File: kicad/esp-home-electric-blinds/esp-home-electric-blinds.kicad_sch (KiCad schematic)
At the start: 10 parts, among them J1 AC_IN, J2 Stepper_2_conn, J3 Stepper_2_conn, J4 Conn_01x05, U1 ESP32_mini, U2 TMC2208_Stepper_driver, U3 TMC2208_Stepper_driver

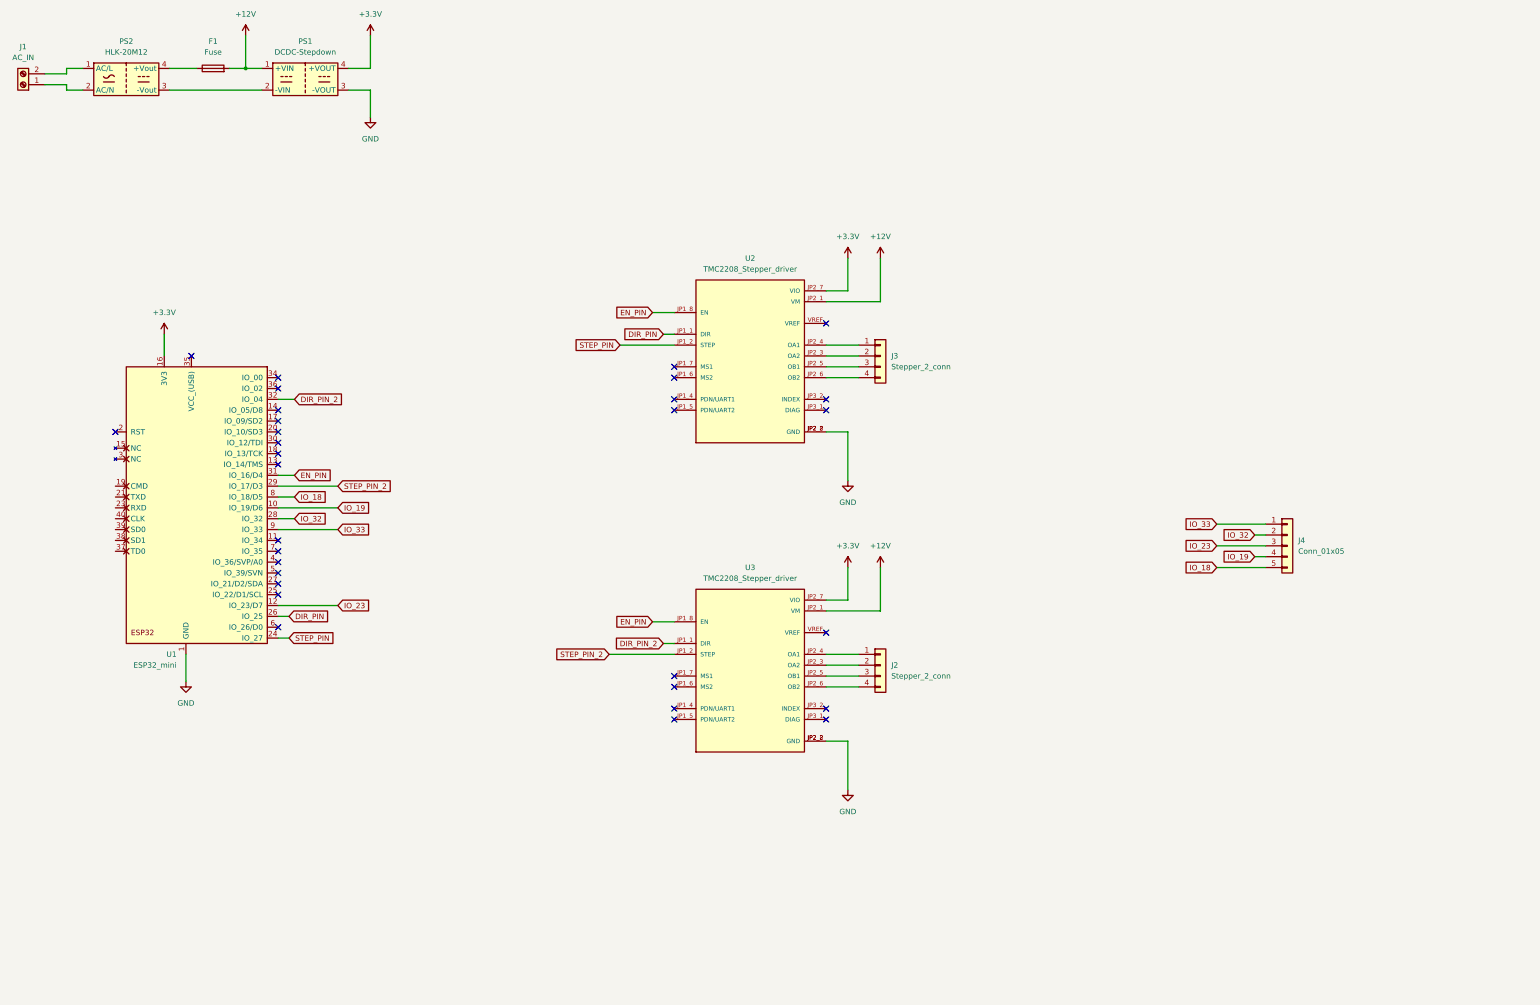
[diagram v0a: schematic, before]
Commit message: rearange
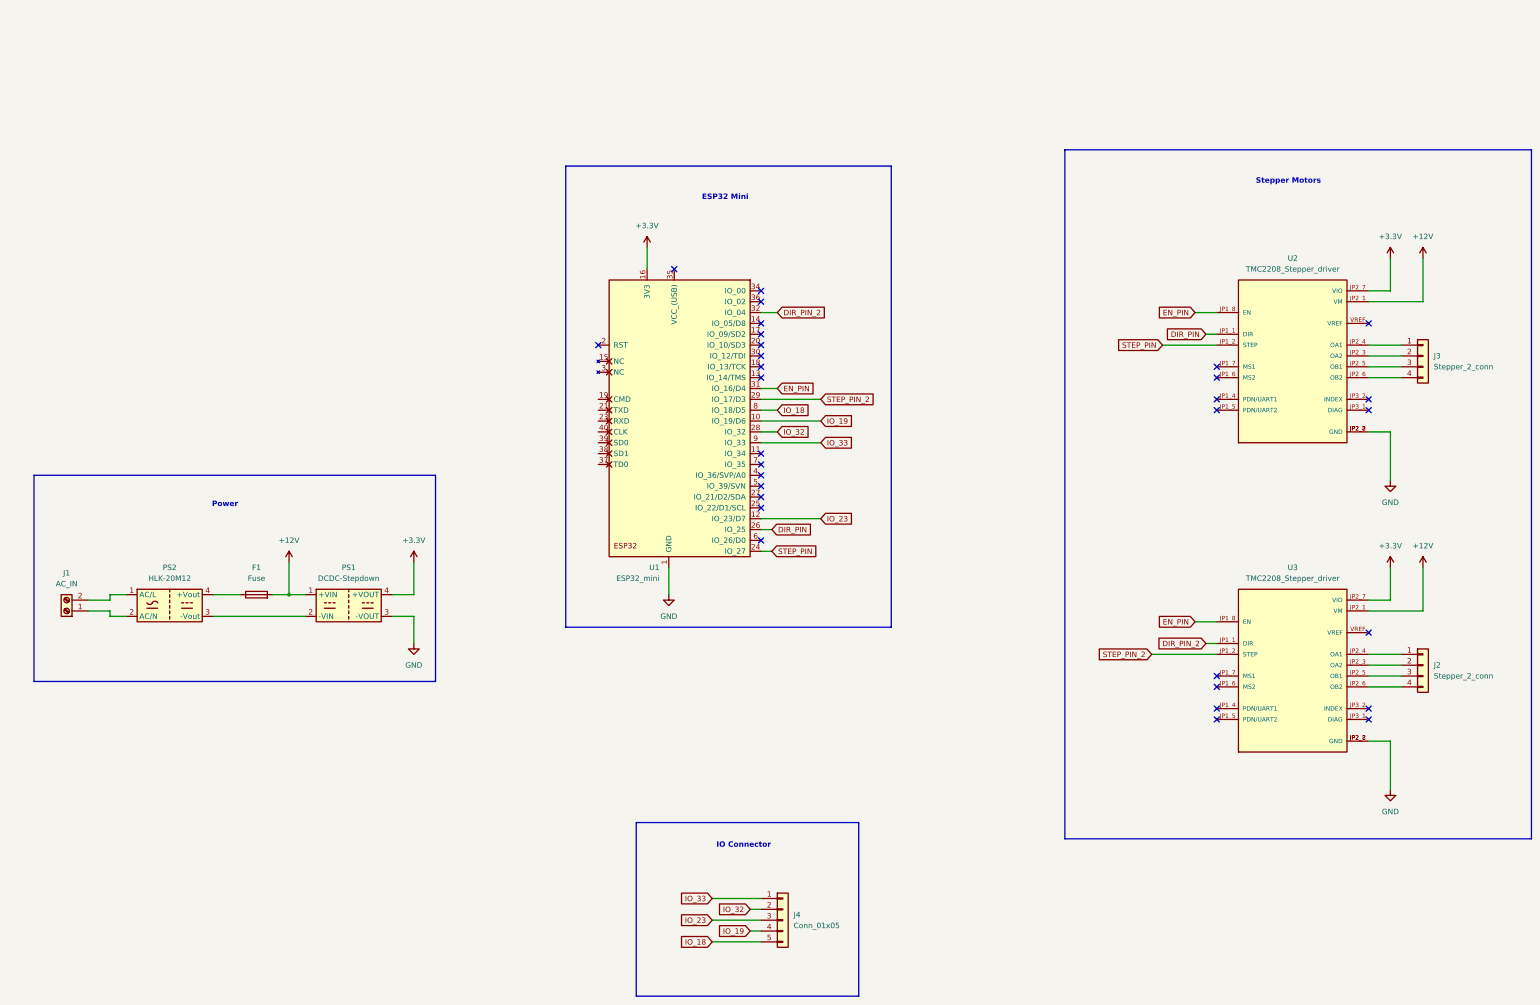
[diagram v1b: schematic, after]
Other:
- note added: "ESP32 Mini"
- note added: "IO Connector"
- note added: "Power"
- note added: "Stepper Motors"
- moved on the sheet: F1, J1, J2, J3, J4, PS1, PS2, U1, U2, U3
